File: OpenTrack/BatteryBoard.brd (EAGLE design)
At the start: 66 x 24 mm, 17 parts, among them U1 POWER-STC4054, U2 POWER-L5980TR, X1 USB-MINIMICROMICRO

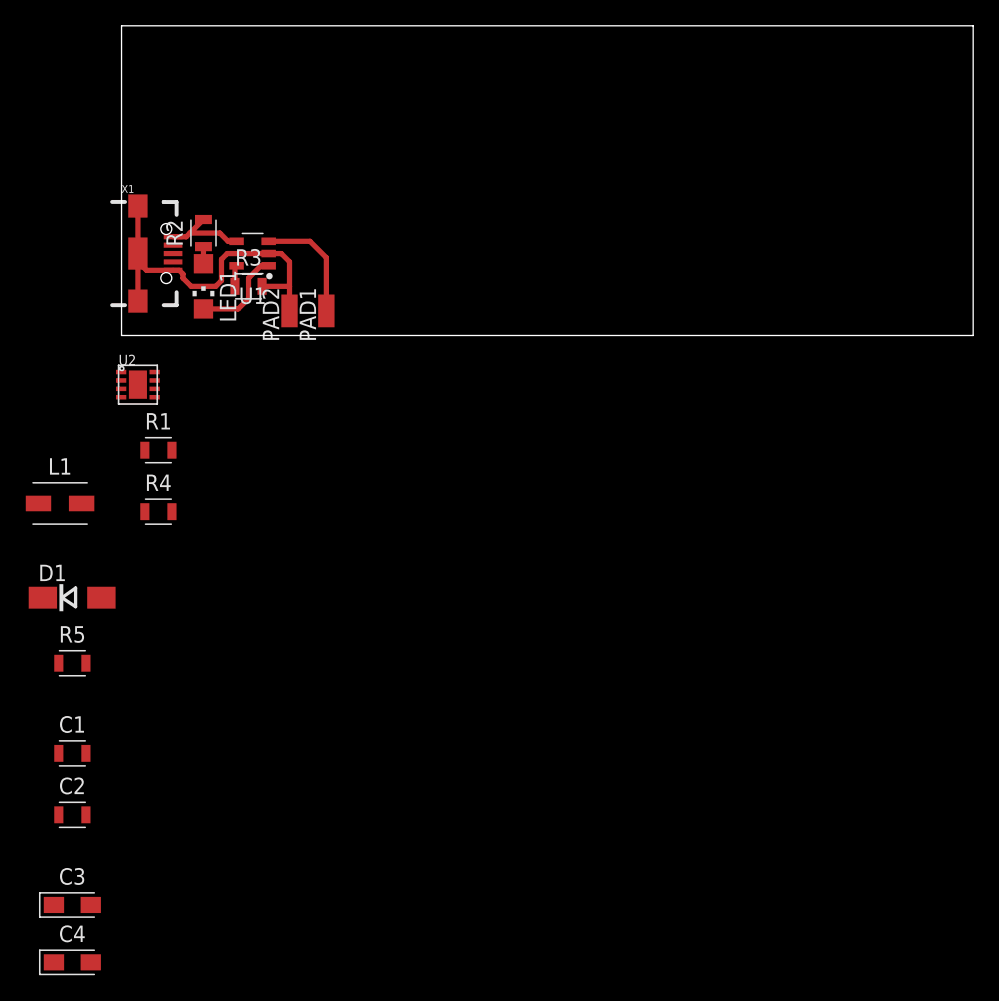
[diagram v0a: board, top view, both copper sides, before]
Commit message: Some Power
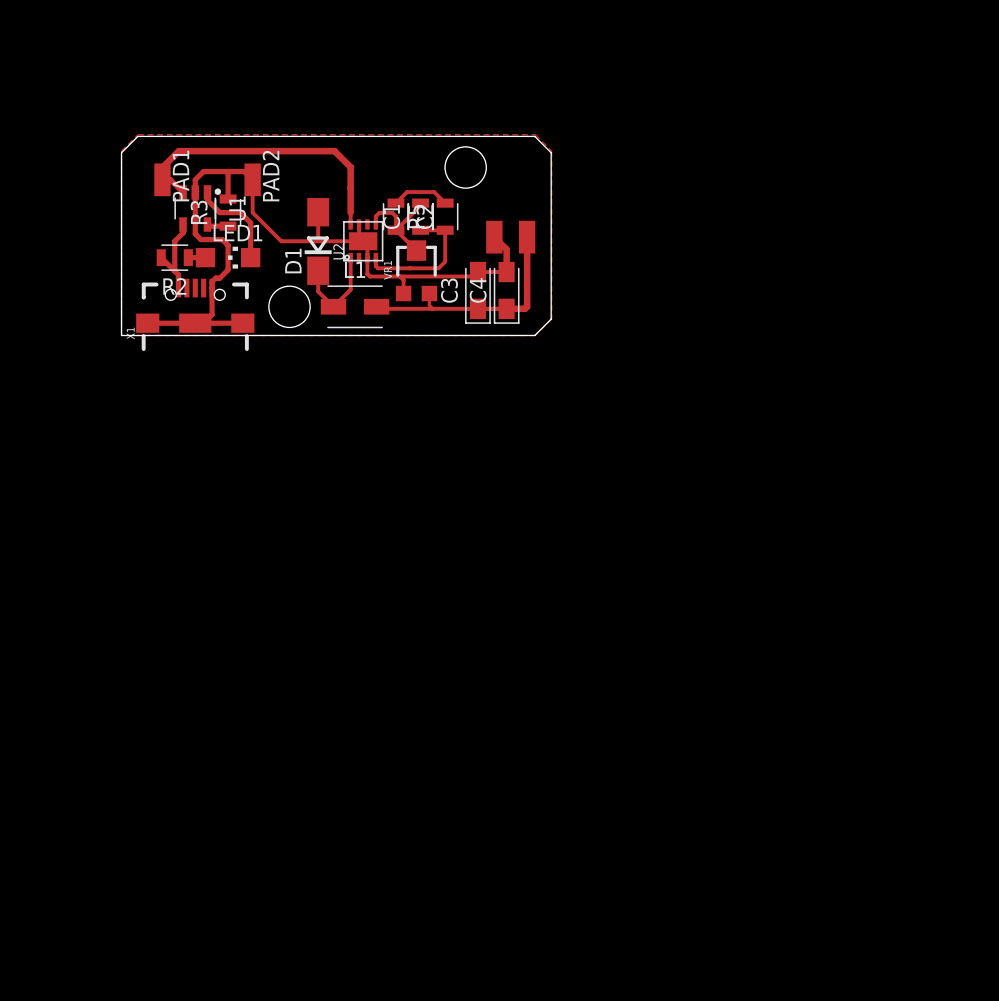
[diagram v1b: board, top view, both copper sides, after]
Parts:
- removed R1, R4: 5K1, Flamberm:RESC2012X50
- added VR1: 10k, SparkFun-Resistors:TRIMPOT-SMD-TC33X
- added X2, X3: (no value), Flamberm:PAD-1.27X2.54
- moved C4 62.0 mm to (29.8, 3.49), turned to 90 degrees
- moved C3 57.1 mm to (27.6, 3.49), turned to 90 degrees
- moved C2 52.7 mm to (21.3, 9.21), turned to 270 degrees
- moved C1 49.6 mm to (23.2, 9.21), turned to 90 degrees
- moved R5 45.1 mm to (25.1, 9.21), turned to 90 degrees
- moved D1 33.6 mm to (15.2, 7.30), turned to 90 degrees
- moved L1 27.5 mm to (18.1, 2.22)
- moved U2 20.7 mm to (18.7, 7.30), turned to 90 degrees
- moved PAD1 16.3 mm to (3.17, 12.1), turned to 180 degrees
- moved PAD2 10.6 mm to (10.2, 12.1), turned to 180 degrees
- moved X1 6.99 mm to (5.71, 0.95), turned to 90 degrees
- moved R3 5.93 mm to (8.26, 9.53), turned to 90 degrees
- moved U1 5.65 mm to (5.71, 9.84), turned to 270 degrees
- moved LED1 2.93 mm to (8.26, 6.03), turned to 270 degrees
- moved R2 2.93 mm to (4.13, 6.03), turned to 180 degrees
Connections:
- net 1V2: now also VR1.3, X2.P$1; no longer R1.1
- net GND: now also VR1.1, X3.P$1; no longer R4.2
- net N$6: now also VR1.2; no longer R1.2, R4.1
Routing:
- net GND: track 28.9 -> 64.2 mm
- net 1V2: track 0.00 -> 21.5 mm
- net V+: track 9.13 -> 23.0 mm
- net N$8: track 0.00 -> 10.6 mm
- net N$6: track 0.00 -> 8.82 mm
- net N$3: track 0.00 -> 7.62 mm
- net N$7: track 0.00 -> 4.52 mm
- added copper zone on layer 1, net GND
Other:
- board size 66 x 24 mm -> 33.3 x 15.4 mm
